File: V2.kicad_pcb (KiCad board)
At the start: 2 copper layers, 50 x 65 mm, 27 parts, among them J1 RFID_Conn, J2 Connections, J3 IR_SENSOR, J4 SERVO, J5 GND, J6 5V, J7 PWR

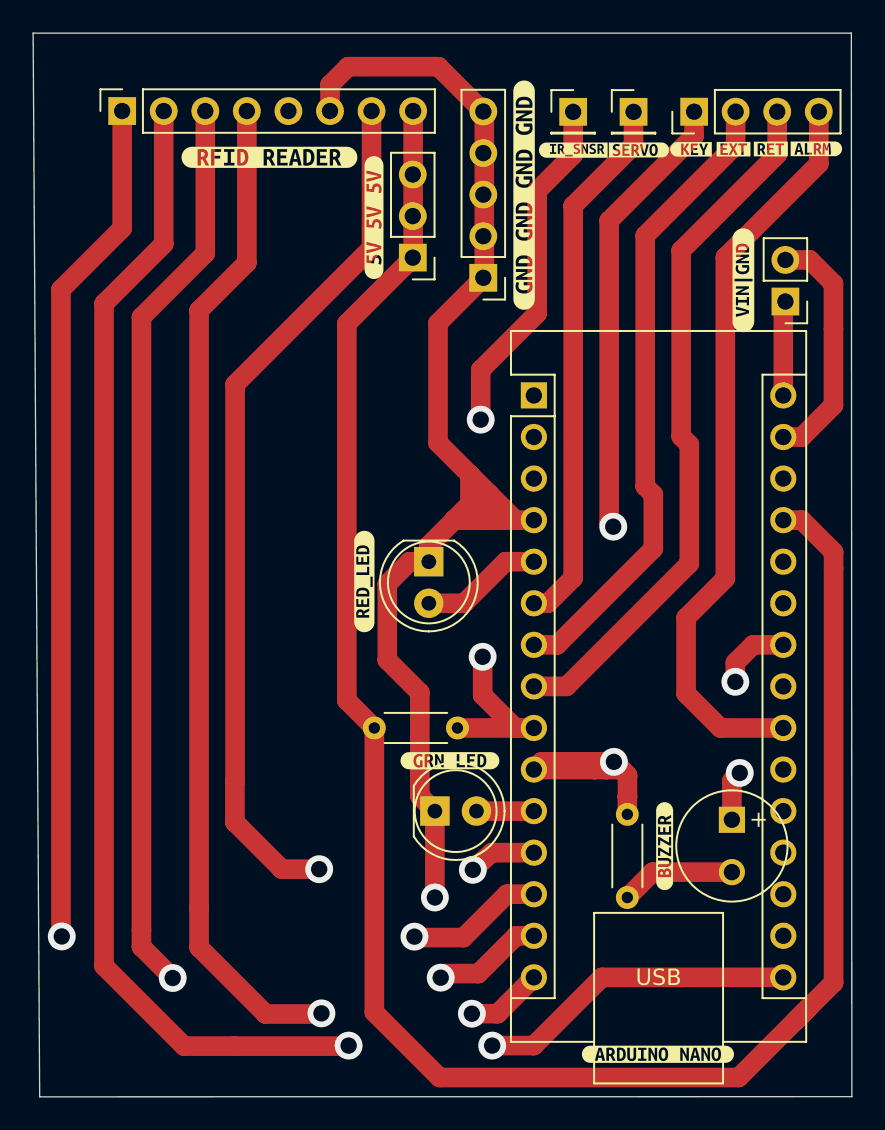
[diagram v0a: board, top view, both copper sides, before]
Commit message: Hardware design files in KiCad
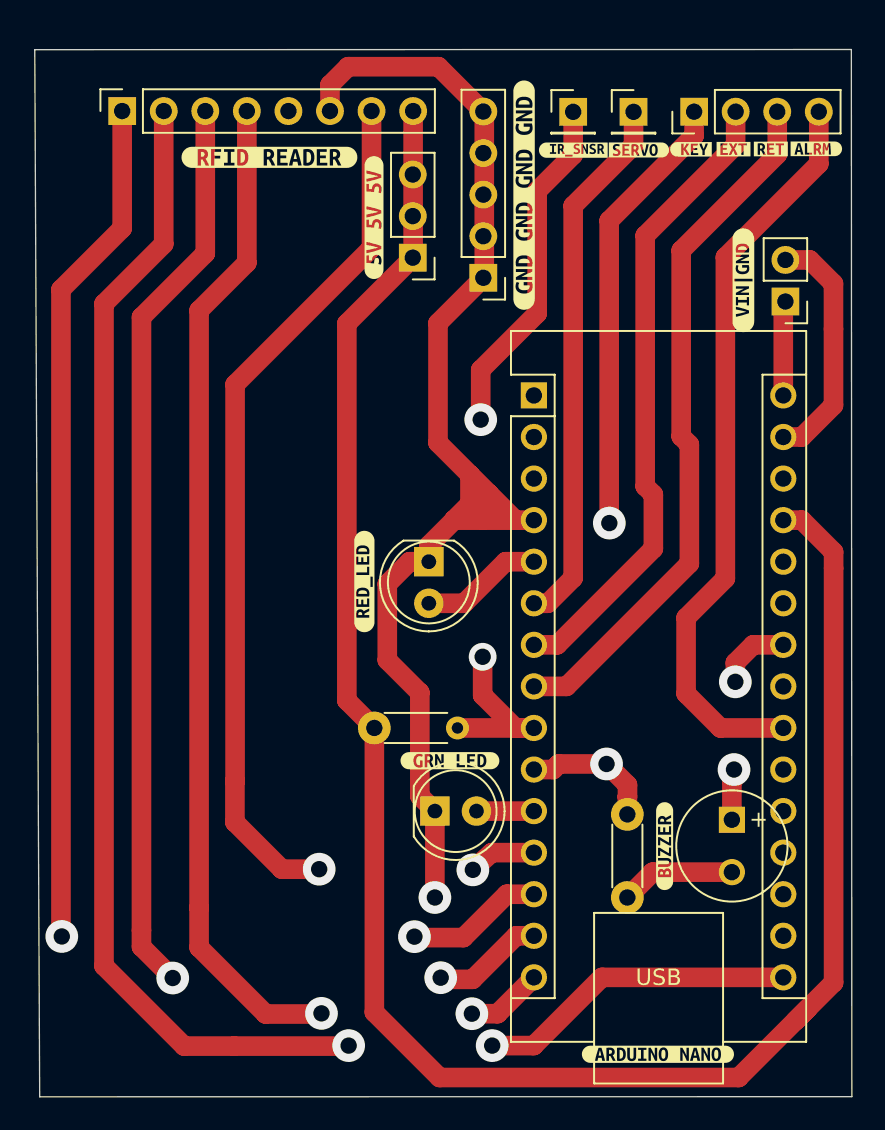
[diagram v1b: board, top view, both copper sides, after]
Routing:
- net KEY_PIN: track 44.2 -> 35.5 mm
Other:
- board size 50 x 65 mm -> 49.9 x 64 mm
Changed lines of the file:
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@@
 			(pintype "passive")
 		)
-		(pad "2" thru_hole oval
+		(pad "2" thru_hole circle
 			(at 5.08 0 180)
-			(size 1.4 1.4)
-			(drill 0.7)
+			(size 2 2)
+			(drill 1)
 			(layers "*.Cu" "*.Mask")
 			(remove_unused_layers no)
@@
 		(pad "1" thru_hole circle
 			(at 0 0 270)
-			(size 1.4 1.4)
-			(drill 0.7)
+			(size 2 2)
+			(drill 1)
 			(layers "*.Cu" "*.Mask")
 			(remove_unused_layers no)
@@
 			(pintype "passive")
 		)
-		(pad "2" thru_hole oval
+		(pad "2" thru_hole circle
 			(at 5.08 0 270)
-			(size 1.4 1.4)
-			(drill 0.7)
+			(size 2 2)
+			(drill 1)
 			(layers "*.Cu" "*.Mask")
 			(remove_unused_layers no)
@@
 	)
 	(gr_line
-		(start 99 79)
-		(end 149 79)
+		(start 99.1 80.01)
+		(end 149 80)
 		(stroke
 			(width 0.05)
@@
 	)
 	(gr_line
-		(start 149 79)
+		(start 149 80)
 		(end 149.03 143.99)
 		(stroke
@@
 	(gr_line
 		(start 99.4 144)
-		(end 99 79)
+		(end 99.1 80.01)
 		(stroke
 			(width 0.05)
@@
 		(layer "Edge.Cuts")
 		(pts
+			(xy 99.4 144) (xy 149.03 143.99)
+		)
+		(height 3.939043)
+		(gr_text "49.6300 mm"
+			(at 124.215562 146.784043 0.01154458568)
+			(layer "Edge.Cuts")
+			(effects
+				(font
+					(size 1 1)
+					(thickness 0.15)
+				)
+			)
+		)
+		(format
+			(prefix "")
+			(suffix "")
+			(units 3)
+			(units_format 1)
+			(precision 4)
+		)
+		(style
+			(thickness 0.05)
+			(arrow_length 1.27)
+			(text_position_mode 0)
+			(extension_height 0.58642)
+			(extension_offset 0.5) keep_text_aligned)
+	)
+	(dimension
+		(type aligned)
+		(layer "Edge.Cuts")
+		(pts
 			(xy 149 79) (xy 124 79)
 		)
@@
 			(extension_offset 0.5) keep_text_aligned)
 	)
+	(dimension
+		(type aligned)
+		(layer "Edge.Cuts")
+		(pts
+			(xy 149 80) (xy 149.03 143.99)
+		)
+		(height -6.836634)
+		(gr_text "63.9900 mm"
+			(at 157.001633 111.991256 270.0268616)
+			(layer "Edge.Cuts")
+			(effects
+				(font
+					(size 1 1)
+					(thickness 0.15)
+				)
+			)
+		)
+		(format
+			(prefix "")
+			(suffix "")
+			(units 3)
+			(units_format 1)
+			(precision 4)
+		)
+		(style
+			(thickness 0.05)
+			(arrow_length 1.27)
+			(text_position_mode 0)
+			(extension_height 0.58642)
+			(extension_offset 0.5) keep_text_aligned)
+	)
 	(segment
 		(start 135.31 125.67)
@@
 	)
 	(segment
-		(start 134.49 123.53)
-		(end 130.07 123.53)
-		(width 1.2)
-		(layer "F.Cu")
-		(net 1)
-	)
-	(segment
-		(start 135.32 124.36)
-		(end 134.96 124)
+		(start 134.04 123.66)
+		(end 135.32 124.94)
 		(width 1.2)
 		(layer "F.Cu")
@@
 	)
 	(segment
-		(start 134.96 124)
-		(end 134.02 124)
-		(width 1.2)
-		(layer "F.Cu")
-		(net 1)
-	)
-	(segment
-		(start 135.32 124.36)
+		(start 135.32 124.94)
 		(end 135.32 125.66)
 		(width 1.2)
@@
 	)
 	(segment
-		(start 134.49 123.53)
-		(end 135.32 124.36)
-		(width 1.2)
-		(layer "F.Cu")
-		(net 1)
-	)
-	(segment
 		(start 134.2 90.46127)
 		(end 139.39 85.27127)
@@
 	)
 	(segment
-		(start 134.02 124)
-		(end 134.49 123.53)
-		(width 1.2)
-		(layer "F.Cu")
-		(net 1)
-	)
-	(segment
-		(start 133.3 124)
-		(end 134.02 124)
-		(width 1.2)
-		(layer "F.Cu")
-		(net 1)
-	)
-	(segment
 		(start 135.32 125.66)
 		(end 135.31 125.67)
@@
 	)
 	(segment
-		(start 134.49 123.53)
-		(end 133.77 123.53)
-		(width 1.2)
-		(layer "F.Cu")
-		(net 1)
-	)
-	(segment
-		(start 129.6 124)
-		(end 133.3 124)
-		(width 1.2)
-		(layer "F.Cu")
-		(net 1)
-	)
-	(segment
-		(start 134.45 109.16)
-		(end 134.2 108.91)
+		(start 130.78 124)
+		(end 129.6 124)
 		(width 1.2)
 		(layer "F.Cu")
@@
 	)
 	(segment
-		(start 133.77 123.53)
-		(end 133.3 124)
+		(start 139.39 85.27127)
+		(end 139.39 83.8)
 		(width 1.2)
 		(layer "F.Cu")
@@
 	)
 	(segment
-		(start 139.39 85.27127)
-		(end 139.39 83.8)
+		(start 131.12 123.66)
+		(end 130.78 124)
 		(width 1.2)
 		(layer "F.Cu")
@@
 	)
 	(segment
-		(start 130.07 123.53)
-		(end 129.6 124)
+		(start 134.04 123.66)
+		(end 131.12 123.66)
 		(width 1.2)
 		(layer "F.Cu")
@@
 	)
 	(via
-		(at 134.49 123.53)
-		(size 1.7)
+		(at 134.04 123.66)
+		(size 2)
 		(drill 1)
 		(layers "F.Cu" "B.Cu")
@@
 	)
 	(via
-		(at 134.45 109.16)
-		(size 1.7)
+		(at 134.21 108.94)
+		(size 2)
 		(drill 1)
 		(layers "F.Cu" "B.Cu")
@@
 	(via
 		(at 116.62 138.9)
-		(size 1.7)
+		(size 2)
 		(drill 1)
 		(layers "F.Cu" "B.Cu")
@@
 	(via
 		(at 125.81 138.92)
-		(size 1.7)
+		(size 2)
 		(drill 1)
 		(layers "F.Cu" "B.Cu")
@@
 	)
 	(via
-		(at 142.18 124.21)
-		(size 1.7)
+		(at 141.83 124)
+		(size 2)
 		(drill 1)
 		(layers "F.Cu" "B.Cu")
@@
 	(via
 		(at 141.91 118.64)
-		(size 1.7)
+		(size 2)
 		(drill 1)
 		(layers "F.Cu" "B.Cu")
@@
 	(via
 		(at 126.35 102.62)
-		(size 1.7)
+		(size 2)
 		(drill 1)
 		(layers "F.Cu" "B.Cu")
@@
 	(via
 		(at 116.48 130.09)
-		(size 1.7)
+		(size 2)
 		(drill 1)
 		(layers "F.Cu" "B.Cu")
@@
 	(via
 		(at 125.87 130.13)
-		(size 1.7)
+		(size 2)
 		(drill 1)
 		(layers "F.Cu" "B.Cu")
@@
 	(via
 		(at 118.28 140.87)
-		(size 1.7)
+		(size 2)
 		(drill 1)
 		(layers "F.Cu" "B.Cu")
@@
 	(via
 		(at 127.051482 140.87)
-		(size 1.7)
+		(size 2)
 		(drill 1)
 		(layers "F.Cu" "B.Cu")
@@
 	(via
 		(at 100.75 134.2)
-		(size 1.7)
+		(size 2)
 		(drill 1)
 		(layers "F.Cu" "B.Cu")
@@
 	(via
 		(at 122.3 134.21322)
-		(size 1.7)
+		(size 2)
 		(drill 1)
 		(layers "F.Cu" "B.Cu")
@@
 	)
 	(segment
-		(start 128.516094 134.16)
-		(end 126.206094 136.47)
+		(start 105.62 133.82)
+		(end 105.62 134.83)
 		(width 1.2)
 		(layer "F.Cu")
@@
 	)
 	(segment
-		(start 105.62 133.82)
-		(end 105.62 134.83)
+		(start 124.154822 136.47)
+		(end 123.904822 136.72)
 		(width 1.2)
 		(layer "F.Cu")
@@
 	)
 	(segment
-		(start 124.154822 136.47)
-		(end 123.904822 136.72)
+		(start 128.516094 134.16)
+		(end 125.856094 136.82)
 		(width 1.2)
 		(layer "F.Cu")
@@
 	)
 	(segment
-		(start 126.206094 136.47)
-		(end 124.154822 136.47)
+		(start 129.6 134.16)
+		(end 128.516094 134.16)
 		(width 1.2)
 		(layer "F.Cu")
@@
 	)
 	(segment
+		(start 124.004822 136.82)
+		(end 123.904822 136.72)
+		(width 1.2)
+		(layer "F.Cu")
+		(net 19)
+	)
+	(segment
 		(start 109.52 83.76)
 		(end 109.52 92.45873)
@@
 	)
 	(segment
-		(start 129.6 134.16)
-		(end 128.516094 134.16)
+		(start 125.856094 136.82)
+		(end 124.004822 136.82)
 		(width 1.2)
 		(layer "F.Cu")
@@
 	(via
 		(at 107.53 136.74)
-		(size 1.7)
+		(size 2)
 		(drill 1)
 		(layers "F.Cu" "B.Cu")
@@
 	(via
 		(at 123.904822 136.72)
-		(size 1.7)
+		(size 2)
 		(drill 1)
 		(layers "F.Cu" "B.Cu")
@@
 	(via
 		(at 123.55 131.82)
-		(size 1.7)
+		(size 2)
 		(drill 1)
 		(layers "F.Cu" "B.Cu")
